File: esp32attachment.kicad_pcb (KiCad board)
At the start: 2 copper layers, 157.6 x 60 mm, 36 parts, among them J1 B2B-PH-SM4-TB, J2 B2B-PH-SM4-TB, J3 B2B-PH-SM4-TB, J4 B2B-PH-SM4-TB, J5 B2B-PH-SM4-TB, J6 B2B-PH-SM4-TB, J7 BATTERY_CONNECTOR, Q1 AOD4184A, Q2 AOD4184A, Q3 AOD4184A, Q4 AOD4184A, Q5 AOD4184A, Q6 AOD4184A, U1 ESP32-DEVKIT-V1, U2 PC847, U3 PC827

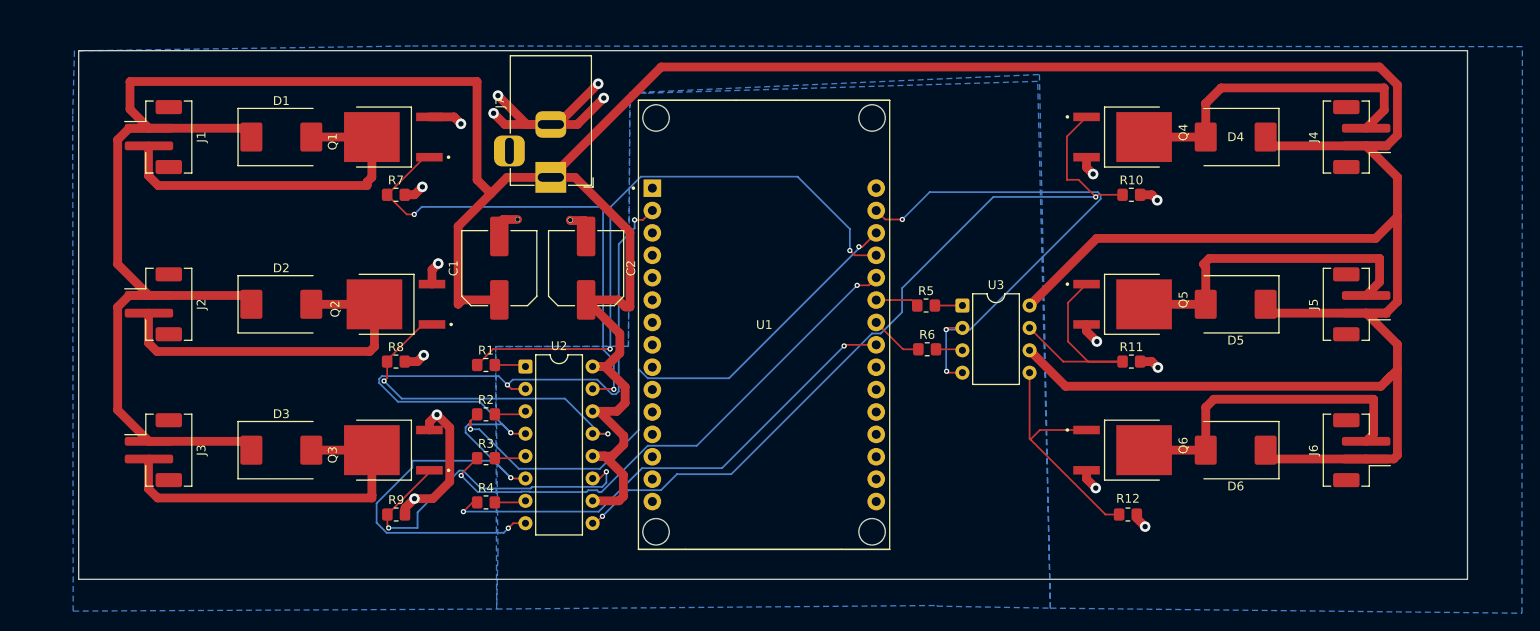
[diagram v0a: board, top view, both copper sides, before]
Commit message: wilkkur review1 changes; still missing mounting holes
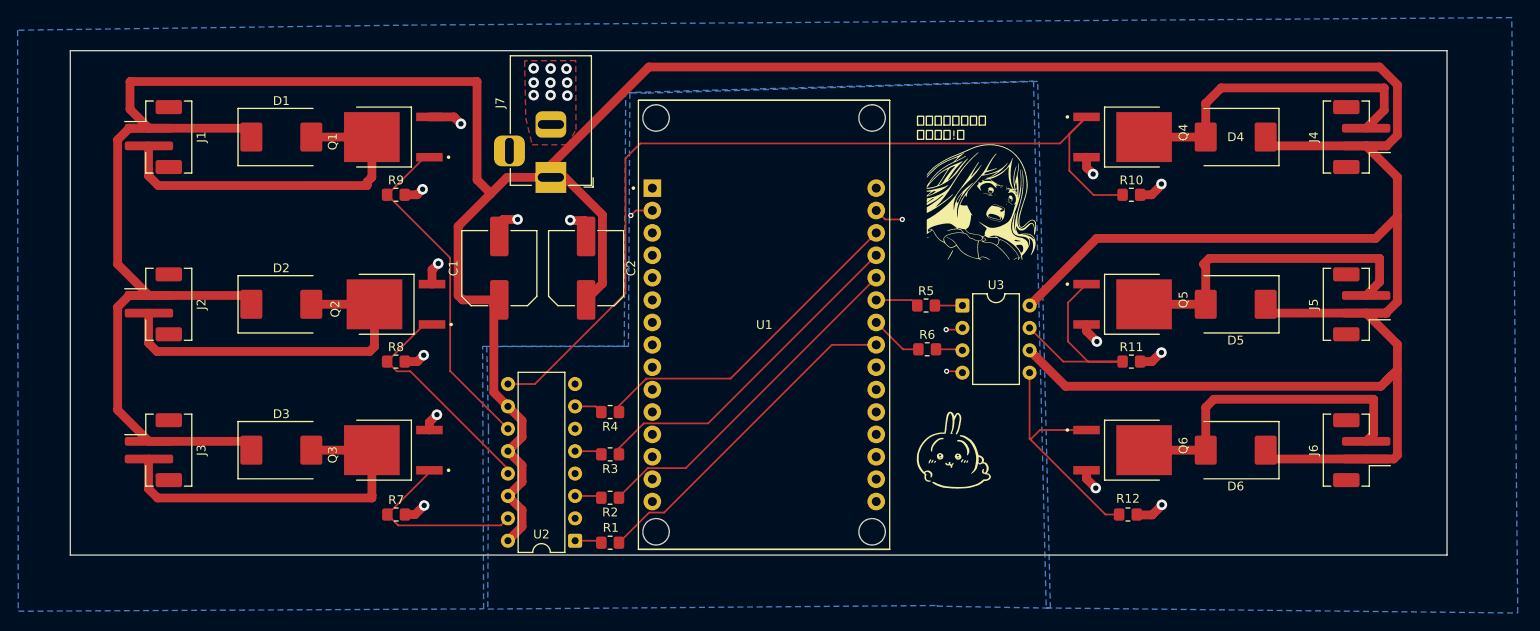
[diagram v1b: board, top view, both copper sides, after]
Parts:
- added G***: LOGO, symbols:usagi, F.Cu at (145.9, 87.6)
- added G***: LOGO, symbols:soyo, F.Cu at (149.9, 59.2)
- moved R7 36.3 mm to (83.0, 94.9)
- moved R9 36.3 mm to (83.0, 58.6)
- moved R1 24.6 mm to (107.2, 98.1), turned to 180 degrees
- moved U2 20.6 mm to (103.3, 97.8), turned to 180 degrees
- moved R4 17.4 mm to (107.2, 83.2), turned to 180 degrees
- moved R2 17.0 mm to (107.2, 93.0), turned to 180 degrees
- moved R3 14.1 mm to (107.2, 88.0), turned to 180 degrees
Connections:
- R1 pad 1: /GPIO12 -> /GPIO25
- R2 pad 1: /GPIO13 -> /GPIO14
- R3 pad 1: /GPIO14 -> /GPIO12
- R4 pad 1: /GPIO25 -> /GPIO13
- R7 pad 1: /FET_GATE1 -> /FET_GATE3
- R9 pad 1: /FET_GATE3 -> /FET_GATE1
- U2 pad 11: /FET_GATE3 -> /FET_GATE1
- U2 pad 15: /FET_GATE1 -> /FET_GATE3
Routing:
- net GND: track 186.8 -> 9.91 mm, vias 8 -> 4
- net GNDPWR: track 78.3 -> 40.3 mm, vias 18 -> 23
- net /GPIO12: track 68.7 -> 39.0 mm, vias 2 -> 0
- net /GPIO13: track 67.0 -> 38.0 mm, vias 2 -> 0
- net /GPIO14: track 60.9 -> 39.6 mm, vias 2 -> 0
- net /FET_GATE3: track 41.3 -> 21.5 mm, vias 2 -> 0
- net /GPIO25: track 56.7 -> 38.5 mm, vias 2 -> 0
- net +12V: track 515.7 -> 498.4 mm
- net /FET_GATE1: track 56.0 -> 38.8 mm, vias 2 -> 0
- net /FET_GATE4: track 89.4 -> 101.3 mm, vias 2 -> 0
- net /FET_GATE2: track 38.9 -> 27.1 mm, vias 2 -> 0
- net Net-(R2-Pad2): track 3.62 -> 3.06 mm
- added copper zone on F.Cu, net GNDPWR
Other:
- board size 157.6 x 60 mm -> 156.2 x 57.2 mm
- board text added: "なんで『春日影』 やったの!？"
